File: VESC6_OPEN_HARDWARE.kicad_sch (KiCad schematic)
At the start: 4 parts

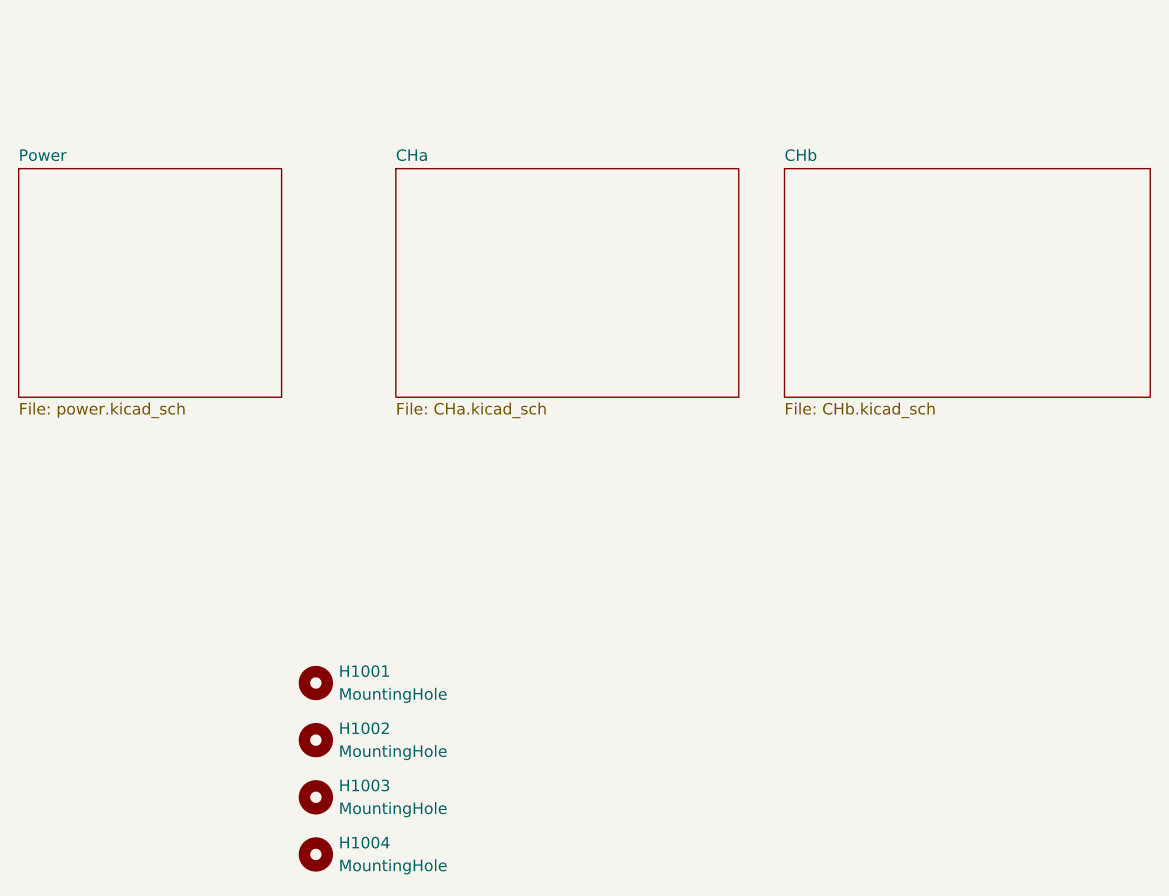
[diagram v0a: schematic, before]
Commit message: it seems to work. yay
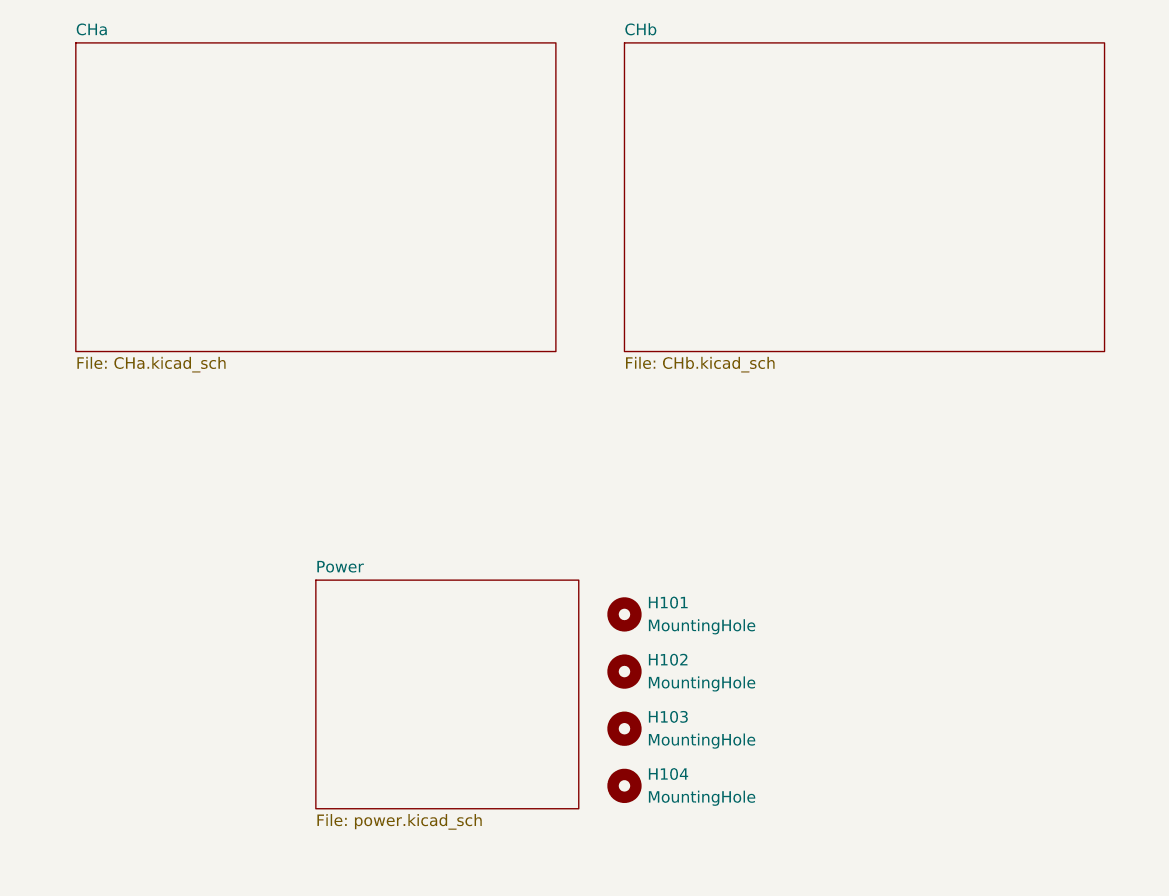
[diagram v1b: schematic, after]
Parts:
- renumbered H1001 to H101, H1002 to H102, H1003 to H103, H1004 to H104
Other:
- moved on the sheet: H101, H102, H103, H104
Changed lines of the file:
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@@
 	(symbol
 		(lib_id "Mechanical:MountingHole")
-		(at 109.22 113.03 0)
+		(at 143.51 105.41 0)
 		(unit 1)
 		(body_style 1)
@@
 		(dnp no)
 		(fields_autoplaced yes)
-		(property "Reference" "H1001"
-			(at 111.76 111.7599 0)
+		(property "Reference" "H101"
+			(at 146.05 104.1399 0)
 			(show_name no)
 			(do_not_autoplace no)
@@
 		)
 		(property "Value" "MountingHole"
-			(at 111.76 114.2999 0)
+			(at 146.05 106.6799 0)
 			(show_name no)
 			(do_not_autoplace no)
@@
 		)
 		(property "Footprint" "CustomFootprints:MountingHole_3mm"
-			(at 109.22 113.03 0)
+			(at 143.51 105.41 0)
 			(hide yes)
 			(show_name no)
@@
 		)
 		(property "Datasheet" ""
-			(at 109.22 113.03 0)
+			(at 143.51 105.41 0)
 			(hide yes)
 			(show_name no)
@@
 		)
 		(property "Description" "Mounting Hole without connection"
-			(at 109.22 113.03 0)
-			(hide yes)
-			(show_name no)
-			(do_not_autoplace no)
-			(effects
-				(font
-					(size 1.27 1.27)
-				)
-			)
-		)
-		(instances
-			(project "VESC6_OPEN_HARDWARE"
-				(path "/8bc2c25a-a1f1-4ce8-b96a-a4f8f4c35079"
-					(reference "H1001")
+			(at 143.51 105.41 0)
+			(hide yes)
+			(show_name no)
+			(do_not_autoplace no)
+			(effects
+				(font
+					(size 1.27 1.27)
+				)
+			)
+		)
+		(instances
+			(project "VESC6_OPEN_HARDWARE"
+				(path "/8bc2c25a-a1f1-4ce8-b96a-a4f8f4c35079"
+					(reference "H101")
 					(unit 1)
 				)
@@
 	(symbol
 		(lib_id "Mechanical:MountingHole")
-		(at 109.22 119.38 0)
+		(at 143.51 111.76 0)
 		(unit 1)
 		(body_style 1)
@@
 		(dnp no)
 		(fields_autoplaced yes)
-		(property "Reference" "H1002"
-			(at 111.76 118.1099 0)
+		(property "Reference" "H102"
+			(at 146.05 110.4899 0)
 			(show_name no)
 			(do_not_autoplace no)
@@
 		)
 		(property "Value" "MountingHole"
-			(at 111.76 120.6499 0)
+			(at 146.05 113.0299 0)
 			(show_name no)
 			(do_not_autoplace no)
@@
 		)
 		(property "Footprint" "CustomFootprints:MountingHole_3mm"
-			(at 109.22 119.38 0)
+			(at 143.51 111.76 0)
 			(hide yes)
 			(show_name no)
@@
 		)
 		(property "Datasheet" ""
-			(at 109.22 119.38 0)
+			(at 143.51 111.76 0)
 			(hide yes)
 			(show_name no)
@@
 		)
 		(property "Description" "Mounting Hole without connection"
-			(at 109.22 119.38 0)
-			(hide yes)
-			(show_name no)
-			(do_not_autoplace no)
-			(effects
-				(font
-					(size 1.27 1.27)
-				)
-			)
-		)
-		(instances
-			(project "VESC6_OPEN_HARDWARE"
-				(path "/8bc2c25a-a1f1-4ce8-b96a-a4f8f4c35079"
-					(reference "H1002")
+			(at 143.51 111.76 0)
+			(hide yes)
+			(show_name no)
+			(do_not_autoplace no)
+			(effects
+				(font
+					(size 1.27 1.27)
+				)
+			)
+		)
+		(instances
+			(project "VESC6_OPEN_HARDWARE"
+				(path "/8bc2c25a-a1f1-4ce8-b96a-a4f8f4c35079"
+					(reference "H102")
 					(unit 1)
 				)
@@
 	(symbol
 		(lib_id "Mechanical:MountingHole")
-		(at 109.22 132.08 0)
+		(at 143.51 124.46 0)
 		(unit 1)
 		(body_style 1)
@@
 		(dnp no)
 		(fields_autoplaced yes)
-		(property "Reference" "H1004"
-			(at 111.76 130.8099 0)
+		(property "Reference" "H104"
+			(at 146.05 123.1899 0)
 			(show_name no)
 			(do_not_autoplace no)
@@
 		)
 		(property "Value" "MountingHole"
-			(at 111.76 133.3499 0)
+			(at 146.05 125.7299 0)
 			(show_name no)
 			(do_not_autoplace no)
@@
 		)
 		(property "Footprint" "CustomFootprints:MountingHole_3mm"
-			(at 109.22 132.08 0)
+			(at 143.51 124.46 0)
 			(hide yes)
 			(show_name no)
@@
 		)
 		(property "Datasheet" ""
-			(at 109.22 132.08 0)
+			(at 143.51 124.46 0)
 			(hide yes)
 			(show_name no)
@@
 		)
 		(property "Description" "Mounting Hole without connection"
-			(at 109.22 132.08 0)
-			(hide yes)
-			(show_name no)
-			(do_not_autoplace no)
-			(effects
-				(font
-					(size 1.27 1.27)
-				)
-			)
-		)
-		(instances
-			(project "VESC6_OPEN_HARDWARE"
-				(path "/8bc2c25a-a1f1-4ce8-b96a-a4f8f4c35079"
-					(reference "H1004")
+			(at 143.51 124.46 0)
+			(hide yes)
+			(show_name no)
+			(do_not_autoplace no)
+			(effects
+				(font
+					(size 1.27 1.27)
+				)
+			)
+		)
+		(instances
+			(project "VESC6_OPEN_HARDWARE"
+				(path "/8bc2c25a-a1f1-4ce8-b96a-a4f8f4c35079"
+					(reference "H104")
 					(unit 1)
 				)
@@
 	(symbol
 		(lib_id "Mechanical:MountingHole")
-		(at 109.22 125.73 0)
+		(at 143.51 118.11 0)
 		(unit 1)
 		(body_style 1)
@@
 		(dnp no)
 		(fields_autoplaced yes)
-		(property "Reference" "H1003"
-			(at 111.76 124.4599 0)
+		(property "Reference" "H103"
+			(at 146.05 116.8399 0)
 			(show_name no)
 			(do_not_autoplace no)
@@
 		)
 		(property "Value" "MountingHole"
-			(at 111.76 126.9999 0)
+			(at 146.05 119.3799 0)
 			(show_name no)
 			(do_not_autoplace no)
@@
 		)
 		(property "Footprint" "CustomFootprints:MountingHole_3mm"
-			(at 109.22 125.73 0)
+			(at 143.51 118.11 0)
 			(hide yes)
 			(show_name no)
@@
 		)
 		(property "Datasheet" ""
-			(at 109.22 125.73 0)
+			(at 143.51 118.11 0)
 			(hide yes)
 			(show_name no)
@@
 		)
 		(property "Description" "Mounting Hole without connection"
-			(at 109.22 125.73 0)
-			(hide yes)
-			(show_name no)
-			(do_not_autoplace no)
-			(effects
-				(font
-					(size 1.27 1.27)
-				)
-			)
-		)
-		(instances
-			(project "VESC6_OPEN_HARDWARE"
-				(path "/8bc2c25a-a1f1-4ce8-b96a-a4f8f4c35079"
-					(reference "H1003")
+			(at 143.51 118.11 0)
+			(hide yes)
+			(show_name no)
+			(do_not_autoplace no)
+			(effects
+				(font
+					(size 1.27 1.27)
+				)
+			)
+		)
+		(instances
+			(project "VESC6_OPEN_HARDWARE"
+				(path "/8bc2c25a-a1f1-4ce8-b96a-a4f8f4c35079"
+					(reference "H103")
 					(unit 1)
 				)
@@
 	)
 	(sheet
-		(at 118.11 55.88)
-		(size 38.1 25.4)
+		(at 82.55 41.91)
+		(size 53.34 34.29)
 		(exclude_from_sim no)
 		(in_bom yes)
@@
 		)
 		(property "Sheetname" "CHa"
-			(at 118.11 55.1684 0)
+			(at 82.55 41.1984 0)
 			(show_name no)
 			(do_not_autoplace no)
@@
 		)
 		(property "Sheetfile" "CHa.kicad_sch"
-			(at 118.11 81.8646 0)
+			(at 82.55 76.7846 0)
 			(show_name no)
 			(do_not_autoplace no)
@@
 			(project "VESC6_OPEN_HARDWARE"
 				(path "/8bc2c25a-a1f1-4ce8-b96a-a4f8f4c35079"
-					(page "9")
+					(page "3")
 				)
 			)
@@
 	)
 	(sheet
-		(at 76.2 55.88)
+		(at 109.22 101.6)
 		(size 29.21 25.4)
 		(exclude_from_sim no)
@@
 		)
 		(property "Sheetname" "Power"
-			(at 76.2 55.1684 0)
+			(at 109.22 100.8884 0)
 			(show_name no)
 			(do_not_autoplace no)
@@
 		)
 		(property "Sheetfile" "power.kicad_sch"
-			(at 76.2 81.8646 0)
+			(at 109.22 127.5846 0)
 			(show_name no)
 			(do_not_autoplace no)
@@
 			(project "VESC6_OPEN_HARDWARE"
 				(path "/8bc2c25a-a1f1-4ce8-b96a-a4f8f4c35079"
-					(page "8")
+					(page "2")
 				)
 			)
@@
 	)
 	(sheet
-		(at 161.29 55.88)
-		(size 40.64 25.4)
+		(at 143.51 41.91)
+		(size 53.34 34.29)
 		(exclude_from_sim no)
 		(in_bom yes)
@@
 		)
 		(property "Sheetname" "CHb"
-			(at 161.29 55.1684 0)
+			(at 143.51 41.1984 0)
 			(show_name no)
 			(do_not_autoplace no)
@@
 		)
 		(property "Sheetfile" "CHb.kicad_sch"
-			(at 161.29 81.8646 0)
+			(at 143.51 76.7846 0)
 			(show_name no)
 			(do_not_autoplace no)
@@
 			(project "VESC6_OPEN_HARDWARE"
 				(path "/8bc2c25a-a1f1-4ce8-b96a-a4f8f4c35079"
-					(page "10")
-				)
-			)
+					(page "4")
+				)
+			)
